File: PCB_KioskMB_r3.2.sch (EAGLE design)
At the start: 339 parts, among them CN2 0039301040, IC1 ISL60002DIH325Z-TK, IC18 FT232RL, IC19 MCP6022-I/ST, IC2 SN65HVD12D, IC20 LTC1771EMS8, IC21 LTC1771EMS8, IC3 PIC24FJ256GA110-I/PT, IC4 PIC10F200T-I/OT, IC5 LM75ADP, IC6 24LC32A-I/MS, IC7 PCF2123TS/1-T, IC8 M25P16-VMN6P, IC9 LM3405AXMK/NOPB, J1 DF11-10DP-2DSA(01), J10 CCM03-3504LFT-NR, J13 3-641215-3, J14 3-641215-2, J15 3-641215-4, J16 3-641215-4, J43 3-641215-4, J44 3-641215-4, J45 3-641215-4, J46 3-641215-5, J47 DF11-10DP-2DSA(01), J48 3-641215-2, J49 3-641215-2, J5 3-641215-2, J6 3-641215-2, J7 SS-6566-NF, J8 TSW-108-07-G-D, J9 SS-6566-NF, Q14 TSM9938HEUK+T, Q15 SI4564DY, Q16 CSD87331Q3D, Q17 TSM9938HEUK+T, Q18 SI4564DY, Q19 CSD87331Q3D, Q2 FDC6330L, Q20 IPD30N06S2L-23, Q21 IPD30N06S2L-23, Q22 FDN352AP, Q23 FDN352AP, Q24 BSS138, Q3 SR3.3.TCT, Q4 7B-28.63636MAAJ-T, Q5 FDC6324L, Q6 CM519 32.768KDZF-UT, Q7 SSM6P49NU,LFPZ, Q8 IPD30N06S2L-23, Q9 IPD30N06S2L-23, U1 LTC1955, U2 HRXL-MAXSONAR-WRC-MB7387, U3 ADS1015, U6 TPS43061, U7 TPS43061, U8 TPA3111D1PWP, U9 OPA322SAIDBVT, X1 FH12-10S-0.5S1.00MM, X2 MINI-USB_4P-85-32004-10X

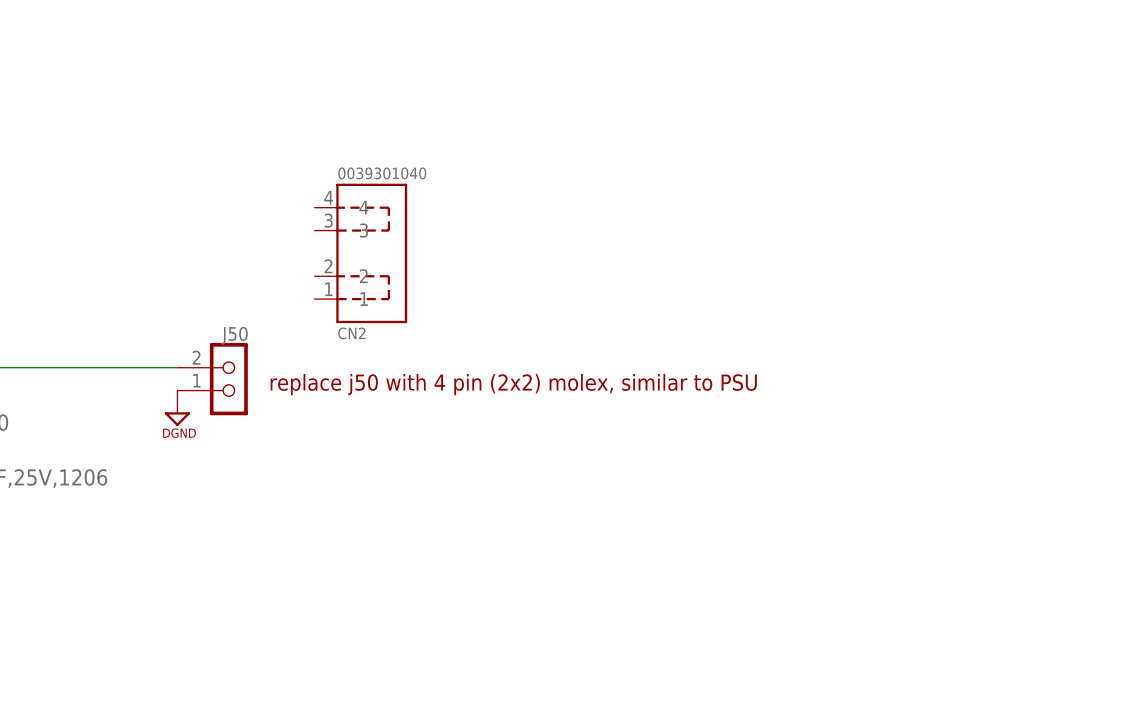
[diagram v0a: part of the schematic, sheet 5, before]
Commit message: push latest
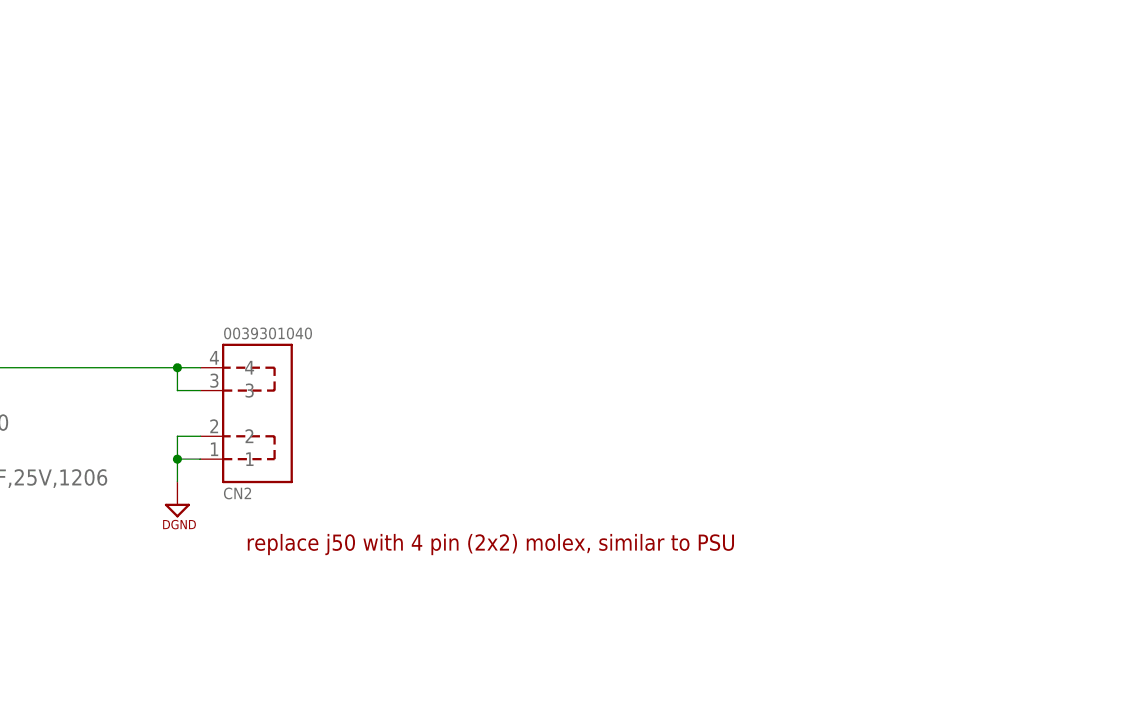
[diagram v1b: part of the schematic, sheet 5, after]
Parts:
- removed J50: (no value), CON-PhoenixContac-AON:TERM-2
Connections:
- net DGND: now also CN2.1, CN2.2; no longer J50.1
- net P12V: now also CN2.3, CN2.4; no longer J50.2
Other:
- moved on the sheet: CN2
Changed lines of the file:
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@@
 <part name="U$342" library="SUPPLY" deviceset="+3.3V/1" device=""/>
 <part name="C187" library="resistor" library_urn="urn:adsk.eagle:library:348" deviceset="CPOL-US" device="E7.5-18" value="2mF/16V"/>
-<part name="J50" library="CON-PhoenixContac-AON" deviceset="TERM-2" device=""/>
 <part name="U$47" library="SUPPLY" deviceset="DGND" device=""/>
 <part name="D32" library="Littelfuse" deviceset="P6SMB*" device="" technology="16A"/>
@@
 <wire x1="40.64" y1="58.42" x2="40.64" y2="60.96" width="0.1524" layer="94"/>
 <wire x1="38.1" y1="78.74" x2="38.1" y2="76.2" width="0.1524" layer="94"/>
-<text x="396.24" y="292.1" size="1.778" layer="94">replace j50 with 4 pin (2x2) molex, similar to PSU</text>
+<text x="393.7" y="274.32" size="1.778" layer="94">replace j50 with 4 pin (2x2) molex, similar to PSU</text>
 </plain>
 <instances>
@@
 <attribute name="VALUE" x="38.735" y="56.8325" size="1.27" layer="96"/>
 </instance>
-<instance part="J50" gate="J" x="391.16" y="294.64" rot="MR0"/>
-<instance part="U$47" gate="G$1" x="386.08" y="289.56" smashed="yes"/>
+<instance part="U$47" gate="G$1" x="386.08" y="279.4" smashed="yes"/>
 <instance part="D32" gate="G$1" x="48.26" y="53.34" smashed="yes" rot="R90">
 <attribute name="NAME" x="47.3075" y="46.7995" size="1.778" layer="95" rot="R90"/>
@@
 </instance>
 <instance part="U$97" gate="G$1" x="447.04" y="241.3" smashed="yes"/>
-<instance part="CN2" gate="G$1" x="406.4" y="307.34" rot="MR180"/>
+<instance part="CN2" gate="G$1" x="393.7" y="289.56" rot="MR180"/>
 </instances>
 <busses>
@@
 <pinref part="D20" gate="G$1" pin="K"/>
 <pinref part="TP61" gate="G$1" pin="TP"/>
-<pinref part="J50" gate="J" pin="2"/>
 <wire x1="360.68" y1="294.64" x2="386.08" y2="294.64" width="0.1524" layer="91"/>
 <junction x="360.68" y="294.64"/>
+<pinref part="CN2" gate="G$1" pin="4"/>
+<pinref part="CN2" gate="G$1" pin="3"/>
+<wire x1="386.08" y1="294.64" x2="388.62" y2="294.64" width="0.1524" layer="91"/>
+<wire x1="388.62" y1="292.1" x2="386.08" y2="292.1" width="0.1524" layer="91"/>
+<wire x1="386.08" y1="292.1" x2="386.08" y2="294.64" width="0.1524" layer="91"/>
+<junction x="386.08" y="294.64"/>
 </segment>
 </net>
@@
 </segment>
 <segment>
-<pinref part="J50" gate="J" pin="1"/>
 <pinref part="U$47" gate="G$1" pin="DGND"/>
+<pinref part="CN2" gate="G$1" pin="2"/>
+<wire x1="388.62" y1="287.02" x2="386.08" y2="287.02" width="0.1524" layer="91"/>
+<wire x1="386.08" y1="287.02" x2="386.08" y2="284.48" width="0.1524" layer="91"/>
+<wire x1="386.08" y1="284.48" x2="386.08" y2="281.94" width="0.1524" layer="91"/>
+<pinref part="CN2" gate="G$1" pin="1"/>
+<wire x1="388.62" y1="284.48" x2="386.08" y2="284.48" width="0.1524" layer="91"/>
+<junction x="386.08" y="284.48"/>
 </segment>
 <segment>
